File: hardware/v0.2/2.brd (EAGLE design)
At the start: 54.9 x 27.5 mm, 36 parts, among them IC1 STM32F10XCXT6, U1 ADXL345"

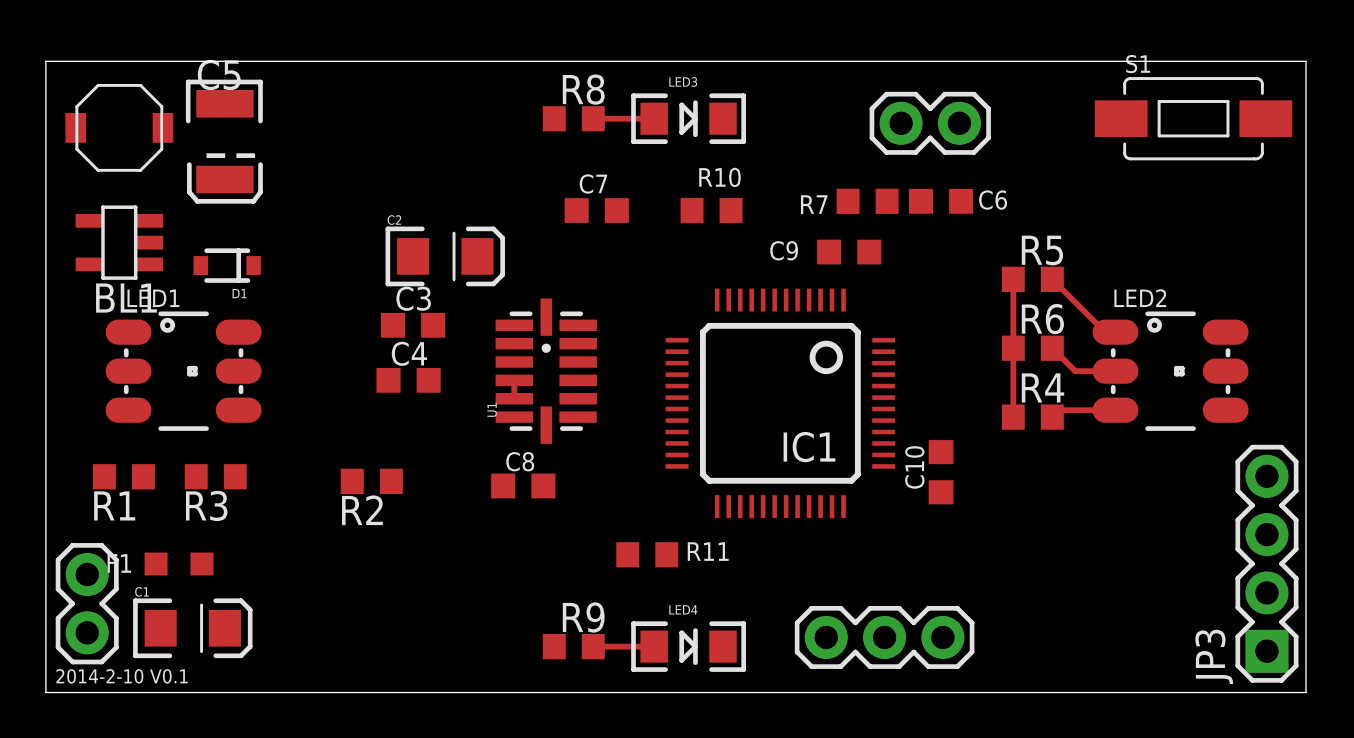
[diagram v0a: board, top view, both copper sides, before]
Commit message: nearly finish PCB design
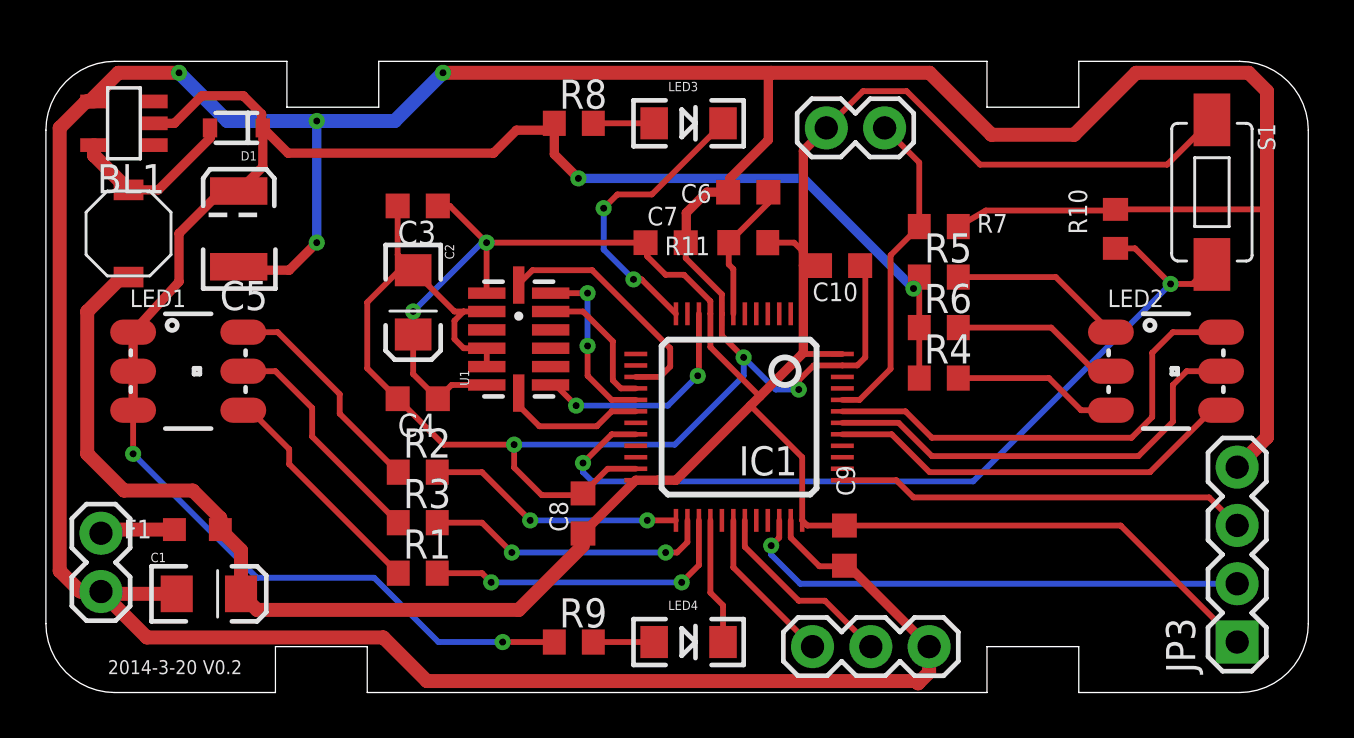
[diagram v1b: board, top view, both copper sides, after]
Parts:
- moved R10 17.6 mm to (46.6, 20.2), turned to 90 degrees
- moved R11 14.3 mm to (30.6, 19.6), turned to 180 degrees
- moved R1 13.5 mm to (16.2, 5.20), turned to 0 degrees
- moved C9 12.8 mm to (34.8, 6.40), turned to 270 degrees
- moved C10 10.0 mm to (34.6, 18.6), turned to 0 degrees
- moved R3 9.02 mm to (16.2, 7.40), turned to 0 degrees
- moved C6 8.41 mm to (30.6, 21.8), turned to 180 degrees
- moved D1 6.01 mm to (8.30, 24.6)
- moved JP4 5.80 mm to (34.0, 24.6), turned to 0 degrees
- moved BL1 5.20 mm to (3.40, 24.8)
- moved C3 5.20 mm to (16.2, 21.2), turned to 180 degrees
- moved L1 4.62 mm to (3.60, 20.0), turned to 90 degrees
- moved R4 4.44 mm to (38.9, 13.7)
- moved R6 4.20 mm to (38.9, 15.9)
- moved R5 4.10 mm to (38.9, 18.1)
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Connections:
- removed net XL345_INT: IC1.13, U1.8
- new net LED3: IC1.12, LED3.C
- new net LED4: IC1.28, LED4.C
- new net N$13: IC1.19
- net 3.3V: now also LED1.1, LED1.2, LED1.3; no longer R1.1, R2.1, R3.1
- net LED1_B: now also IC1.27, R1.2; no longer LED1.4
- net LED1_G: now also IC1.25, R2.2; no longer LED1.6
- net LED1_R: now also IC1.26, R3.2; no longer LED1.5
- net LED2_B: now also IC1.41
- net LED2_G: now also IC1.43
- net LED2_R: now also IC1.42
- net N$6: now also LED1.4, R1.1; no longer LED1.3, R1.2
- net N$7: now also LED1.6, R2.1; no longer LED1.1, R2.2
- net N$8: now also LED1.5, R3.1; no longer LED1.2, R3.2
- net WAKEUP: now also U1.8; no longer U1.9
- net XL345_CS: now also IC1.18; no longer IC1.14
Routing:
- net GND: track 0.80 -> 240.3 mm, vias 0 -> 7
- net 2.8V: track 0.00 -> 144.1 mm, vias 0 -> 2
- net 3.3V: track 6.00 -> 83.6 mm, vias 0 -> 4
- net N$2: track 0.00 -> 37.7 mm, vias 0 -> 2
- net SWDIO: track 0.00 -> 22.5 mm, vias 0 -> 1
- net LED2_G: track 0.00 -> 20.5 mm
- net LED2_R: track 0.00 -> 19.6 mm
- net LED2_B: track 0.00 -> 18.4 mm
- net SWCLK: track 0.00 -> 18.0 mm
- net BOOT0: track 0.00 -> 14.3 mm
- net LED1_B: track 0.00 -> 13.8 mm, vias 0 -> 2
- net LED3: track 0.00 -> 12.8 mm, vias 0 -> 2
- net LED1_R: track 0.00 -> 12.8 mm, vias 0 -> 2
- net LED1_G: track 0.00 -> 11.3 mm, vias 0 -> 2
- net XL345_SCK: track 0.00 -> 10.8 mm
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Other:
- board size 54.9 x 27.5 mm -> 55 x 27.5 mm
- board text added: "2014-3-20 V0.2"
- board text removed: "2014-2-10 V0.1"
